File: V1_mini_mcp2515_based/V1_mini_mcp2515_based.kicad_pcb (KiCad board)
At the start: 2 copper layers, 73.4 x 65.8 mm, 19 parts, among them IC1 MCP2515-I_P, J1 Conn_01x07, J2 Screw_Terminal_01x02, J4 Conn_01x01, J5 Conn_01x05, J6 Conn_01x05, J7 Conn_01x05, J8 Screw_Terminal_01x02, U1 LF50_TO220, Y1 Resonator_Small

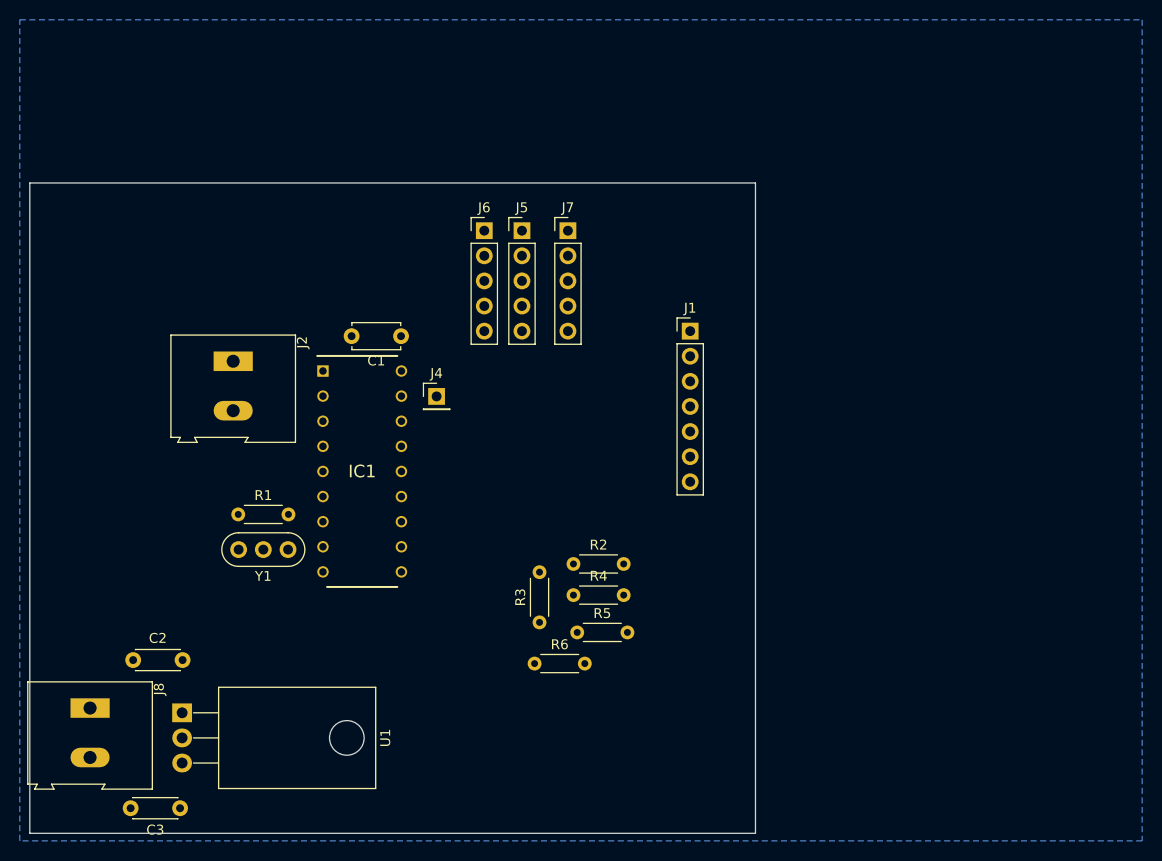
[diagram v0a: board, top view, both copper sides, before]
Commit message: f
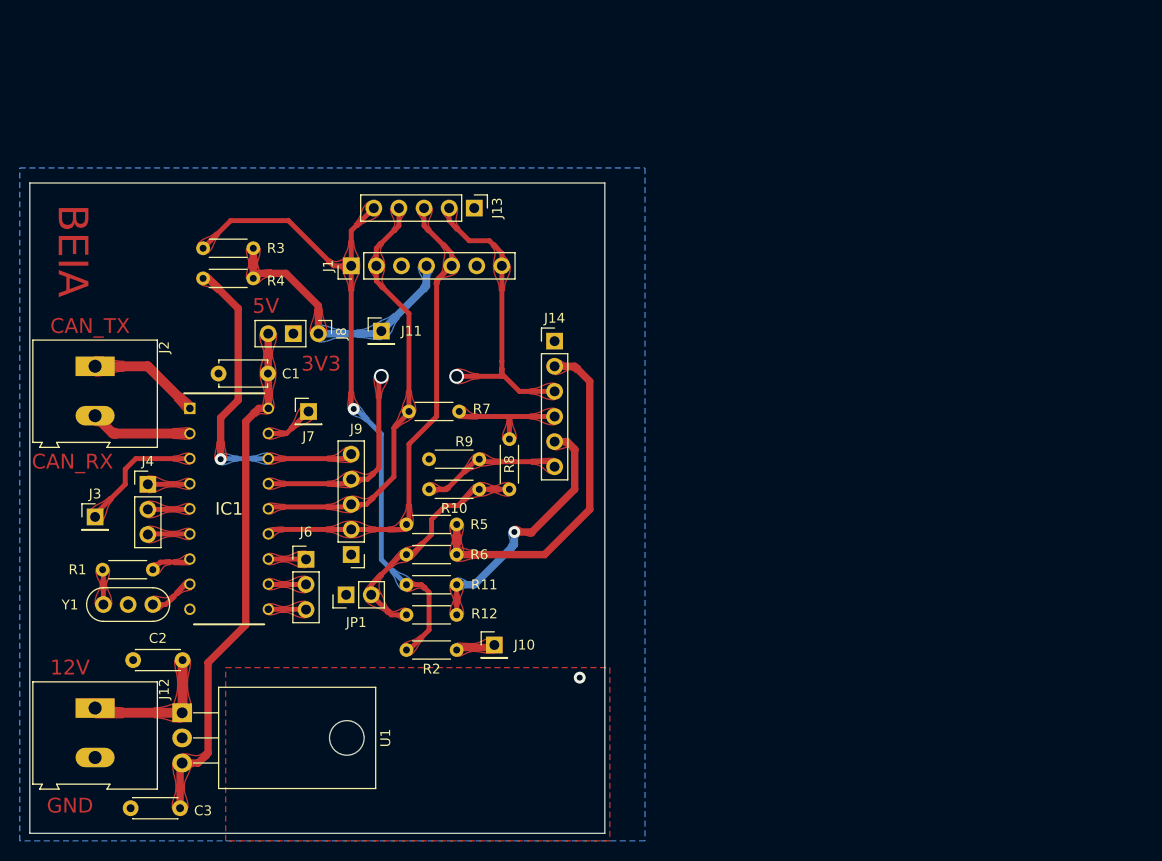
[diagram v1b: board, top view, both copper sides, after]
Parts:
- added J10: Conn_01x01, Connector_PinHeader_2.54mm:PinHeader_1x01_P2.54mm_Vertical, F.Cu at (82.8, 130.6)
- added J11: Conn_01x01, Connector_PinHeader_2.54mm:PinHeader_1x01_P2.54mm_Vertical, F.Cu at (71.4, 98.8)
- added J14: SPI_AVR, Connector_PinHeader_2.54mm:PinHeader_1x06_P2.54mm_Vertical, F.Cu at (88.9, 99.8)
- added J3: Conn_01x01, Connector_PinHeader_2.54mm:PinHeader_1x01_P2.54mm_Vertical, F.Cu at (42.4, 117.6)
- added J4: Conn_01x03, Connector_PinHeader_2.54mm:PinHeader_1x03_P2.54mm_Vertical, F.Cu at (47.8, 114.3)
- added J8: power, Connector_PinHeader_2.54mm:PinHeader_1x03_P2.54mm_Vertical, F.Cu at (65.0, 99.1)
- added JP1: Jumper_2_Open, Connector_PinHeader_2.54mm:PinHeader_1x02_P2.54mm_Vertical, F.Cu at (67.8, 125.5)
- added R10: R_Small, Resistor_THT:R_Axial_DIN0204_L3.6mm_D1.6mm_P5.08mm_Horizontal, F.Cu at (81.3, 114.8)
- added R11: R_Small, Resistor_THT:R_Axial_DIN0204_L3.6mm_D1.6mm_P5.08mm_Horizontal, F.Cu at (79.0, 124.5)
- added R12: R_Small, Resistor_THT:R_Axial_DIN0204_L3.6mm_D1.6mm_P5.08mm_Horizontal, F.Cu at (73.9, 127.5)
- added R7: R_Small, Resistor_THT:R_Axial_DIN0204_L3.6mm_D1.6mm_P5.08mm_Horizontal, F.Cu at (79.2, 106.9)
- added R8: R_Small, Resistor_THT:R_Axial_DIN0204_L3.6mm_D1.6mm_P5.08mm_Horizontal, F.Cu at (84.3, 114.8)
- added R9: R_Small, Resistor_THT:R_Axial_DIN0204_L3.6mm_D1.6mm_P5.08mm_Horizontal, F.Cu at (81.3, 111.8)
- J1: value Conn_01x07 -> SD_crd
- J13: renamed from J7; value Conn_01x05 -> SPI2
- J6: value Conn_01x05 -> Conn_01x03; footprint Connector_PinHeader_2.54mm:PinHeader_1x05_P2.54mm_Vertical -> Connector_PinHeader_2.54mm:PinHeader_1x03_P2.54mm_Vertical
- J9: renamed from J5; value Conn_01x05 -> SPI1
- R2: value R_Small -> 10k
- moved R3 50.8 mm to (58.4, 90.4), turned to 180 degrees
- moved R4 48.2 mm to (58.4, 93.5), turned to 180 degrees
- moved J6 37.8 mm to (63.8, 121.9)
- moved J9 37.0 mm to (68.3, 121.4), turned to 180 degrees
- moved J1 34.9 mm to (68.3, 92.2), turned to 90 degrees
- moved R6 17.4 mm to (73.9, 121.4)
- moved R1 14.8 mm to (43.2, 122.9)
- moved Y1 14.8 mm to (48.3, 126.5)
- moved R2 14.7 mm to (79.0, 131.1), turned to 180 degrees
- moved C1 14.0 mm to (59.9, 103.1)
- moved IC1 14.0 mm to (56.0, 116.8)
- moved J2 14.0 mm to (42.4, 102.4)
- moved J7 13.0 mm to (64.0, 106.9)
- moved R5 13.0 mm to (79.0, 118.4), turned to 180 degrees
- moved J13 9.75 mm to (80.8, 86.4), turned to -90 degrees
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- renumbered J8 to J12, J4 to J7, R5 to R3, R6 to R4, R3 to R5, R4 to R6
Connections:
- IC1 pad 10: unconnected-(IC1-Pad10) -> Net-(IC1-Pad10)
- IC1 pad 11: unconnected-(IC1-Pad11) -> Net-(IC1-Pad11)
- IC1 pad 12: unconnected-(IC1-Pad12) -> Net-(IC1-Pad12)
- IC1 pad 3: unconnected-(IC1-Pad3) -> Net-(IC1-Pad3)
- IC1 pad 4: unconnected-(IC1-Pad4) -> Net-(IC1-Pad4)
- IC1 pad 5: unconnected-(IC1-Pad5) -> Net-(IC1-Pad5)
- IC1 pad 6: unconnected-(IC1-Pad6) -> Net-(IC1-Pad6)
- J1 pad 2: /MOSI -> SPI_MOSI
- J1 pad 5: /CLK -> SPI_CLK
- J1 pad 7: /MISO -> SPI_MISO
- J13 pad 2: /CLK -> SPI_MISO
- J13 pad 3: /MISO -> SPI_CLK
- J13 pad 4: /MOSI -> SPI_MOSI
- J6 pad 1: GND -> Net-(IC1-Pad12)
- J6 pad 2: SPI_CLK -> Net-(IC1-Pad11)
- J6 pad 3: SPI_MOSI -> Net-(IC1-Pad10)
- R5 pad 2: unconnected-(R3-Pad2) -> SPI_CLK
- R6 pad 1: GND -> Net-(JP1-Pad2)
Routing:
- net /SS: track 0.00 -> 69.1 mm, vias 0 -> 1
- net +5V: track 0.00 -> 53.2 mm
- net SPI_MISO: track 0.00 -> 52.8 mm, vias 0 -> 2
- net SPI_CLK: track 0.00 -> 49.4 mm
- net SPI_MOSI: track 0.00 -> 44.2 mm
- net Net-(J14-Pad2): track 0.00 -> 35.5 mm
- net SPI_SS: track 0.00 -> 34.2 mm, vias 0 -> 1
- net +3V3: track 0.00 -> 33.0 mm
- net Net-(J14-Pad5): track 0.00 -> 26.1 mm, vias 0 -> 1
- net Net-(JP1-Pad2): track 0.00 -> 24.3 mm
- net +12V: track 0.00 -> 14.4 mm
- net Net-(J14-Pad6): track 0.00 -> 14.3 mm
- net Net-(IC1-Pad3): track 0.00 -> 13.1 mm
- net Net-(J14-Pad4): track 0.00 -> 12.1 mm
- net Net-(IC1-Pad1): track 0.00 -> 11.4 mm
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- added copper zone on F.Cu, net GND
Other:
- board size 73.4 x 65.8 mm -> 58.2 x 65.8 mm
- board text added: "12V"
- board text added: "3V3"
- board text added: "5V"
- board text added: "BEIA"
- board text added: "CAN_RX"
- board text added: "CAN_TX"
- board text added: "GND"
